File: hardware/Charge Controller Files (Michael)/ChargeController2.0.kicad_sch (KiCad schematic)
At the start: 76 parts, among them J1 Conn_01x02_Pin, J10 Conn-1x2, J11 Conn-1x2, J12 Conn-1x2, J13 Conn-1x2, J14 Conn-1x2, J15 Conn-1x2, J16 Conn-1x2, J2 Conn_01x02_Pin, J3 Conn-1x2, J6 Conn-1x2, J7 Conn-1x2, J8 Conn-1x2, J9 Conn-1x2, Q5 AONS66614, Q6 AONS66614, Q7 AONS66614, Q8 AONS66614, U1 BQ25756RRVR

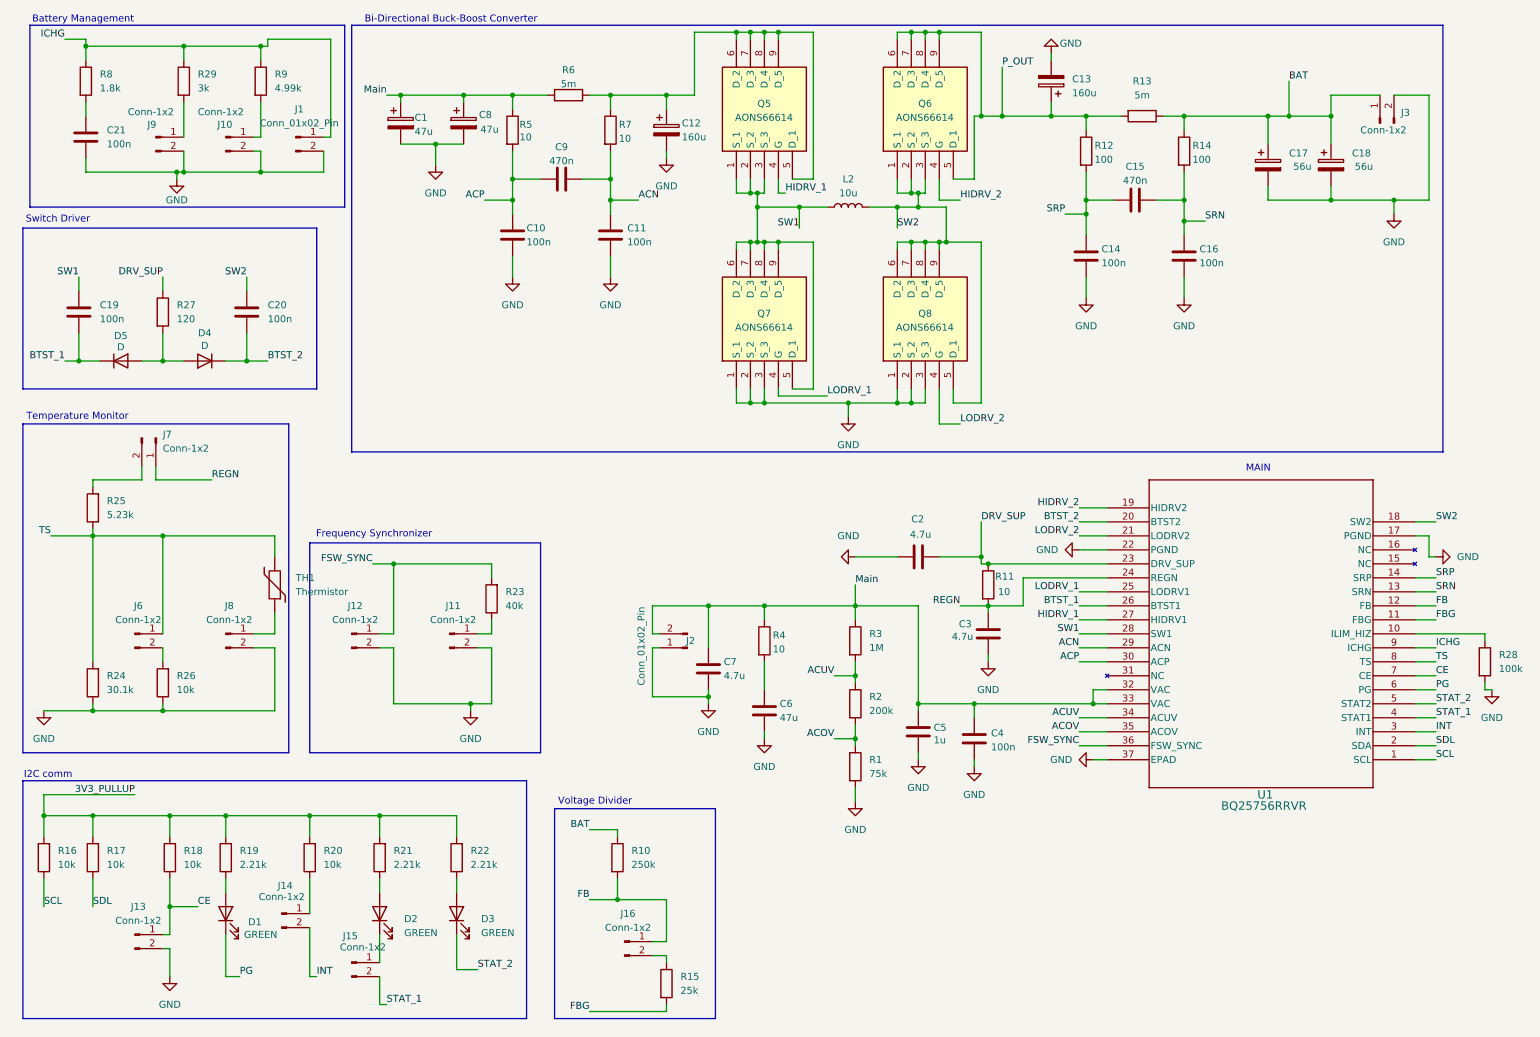
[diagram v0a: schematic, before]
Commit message: Design Specs Update II
Updates Design specs and layout
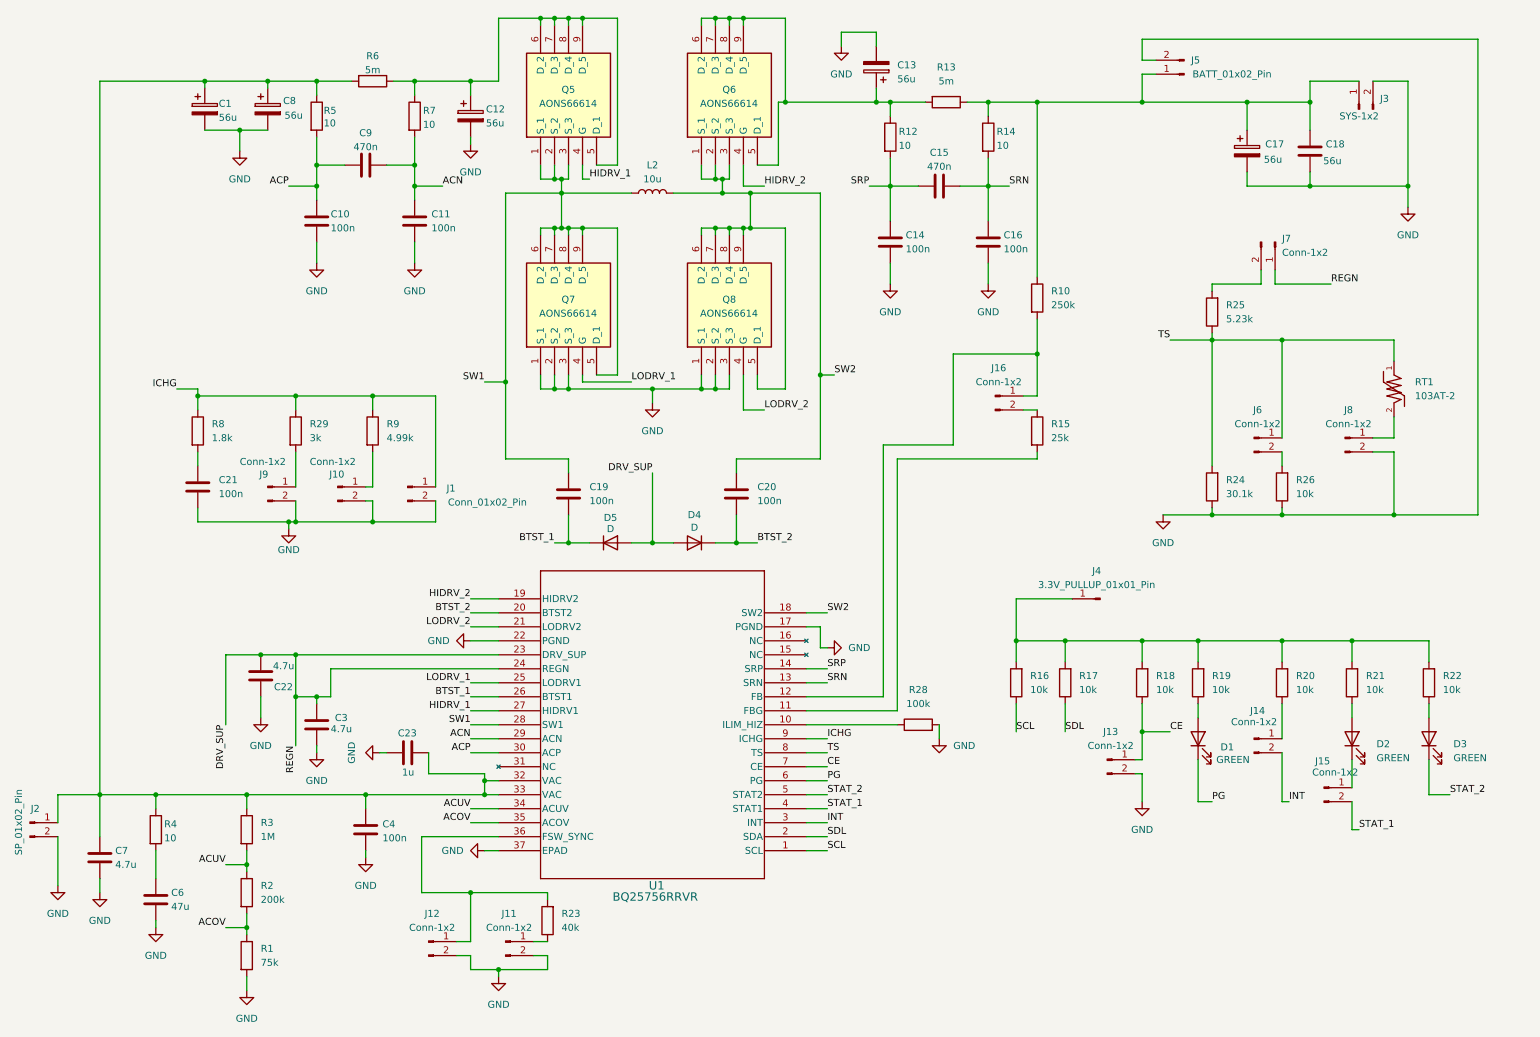
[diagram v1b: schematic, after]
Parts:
- removed C18: 56u, symbol Device:C_Polarized
- removed C2: 4.7u, symbol Device:C
- removed C5: 1u, symbol Device:C
- removed R11: 10, symbol Device:R
- removed R27: 120, symbol Device:R
- removed TH1: Thermistor, symbol Device:Thermistor
- added C18: 56u, symbol Device:C
- added C22: 4.7u, symbol Device:C
- added C23: 1u, symbol Device:C
- added J4: 3.3V_PULLUP_01x01_Pin, symbol Connector:Conn_01x01_Pin
- added J5: BATT_01x02_Pin, symbol Connector:Conn_01x02_Pin
- added RT1: 103AT-2, 103AT-2:103AT-2, symbol 103AT-2:103AT-2
- C1, C8: value 47u -> 56u
- C12, C13: value 160u -> 56u
- J2: value Conn_01x02_Pin -> SP_01x02_Pin
- J3: value Conn-1x2 -> SYS-1x2
- R12, R14: value 100 -> 10
- R19, R21, R22: value 2.21k -> 10k
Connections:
- net REGN is gone; now on net DRV_SUP: C3.1, J7.1 (Pin_1), U1.24 (REGN)
- net DRV_SUP: now also D4.2 (A), D5.2 (A), C22.1
- net GND: now also J2.2 (Pin_2), C18.2, C22.2, C23.2, J5.2 (Pin_2); no longer J2.1 (Pin_1)
- net TS: now also RT1.1
- net at J8.1 (Pin_1): now also RT1.2
- net 3V3_PULLUP: no longer names the net of R16.2, R17.2, R18.2, R19.2, R20.2, R21.2, R22.2
- net 3V3_PULLUP: now also J4.1 (Pin_1)
- net BAT: no longer names the net of C17.1, J3.1 (Pin_1), R10.1, R13.1, R14.1
- net BAT: now also C18.1, J5.1 (Pin_1)
- net FB: no longer names the net of J16.1 (Pin_1), R10.2, U1.12 (FB)
- net FBG: no longer names the net of R15.2, U1.11 (FBG)
- net FSW_SYNC: no longer names the net of J12.1 (Pin_1), R23.2, U1.36 (FSW_SYNC)
- net Main: no longer names the net of C1.1, C4.1, C7.1, C8.1, R3.1, R4.1, R5.1, R6.2, U1.32 (VAC), U1.33 (VAC)
- net Main: now also J2.1 (Pin_1), C23.1; no longer J2.2 (Pin_2)
- net P_OUT: no longer names the net of C13.1, Q6.5 (D_1), Q6.6 (D_2), Q6.7 (D_3), Q6.8 (D_4), Q6.9 (D_5), R12.1, R13.2
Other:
- note removed: "Battery Management"
- note removed: "Bi-Directional Buck-Boost Converter"
- note removed: "Frequency Synchronizer"
- note removed: "I2C comm"
- note removed: "MAIN"
- note removed: "Switch Driver"
- note removed: "Temperature Monitor"
- note removed: "Voltage Divider"
- moved on the sheet: C1, C10, C11, C12, C13, C14, C15, C16, C17, C19, C20, C21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
